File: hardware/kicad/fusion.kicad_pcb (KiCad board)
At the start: 2 copper layers, 32 parts, among them J1 BATTERY, J2 LSM6DSOX, J3 PICKIT, J4 HC-05, J5 FLEX, J7 FTDI, SW1 BUTTON, SW2 POWER, SW3 UART, U1 MCP1603, U2 PIC16F690

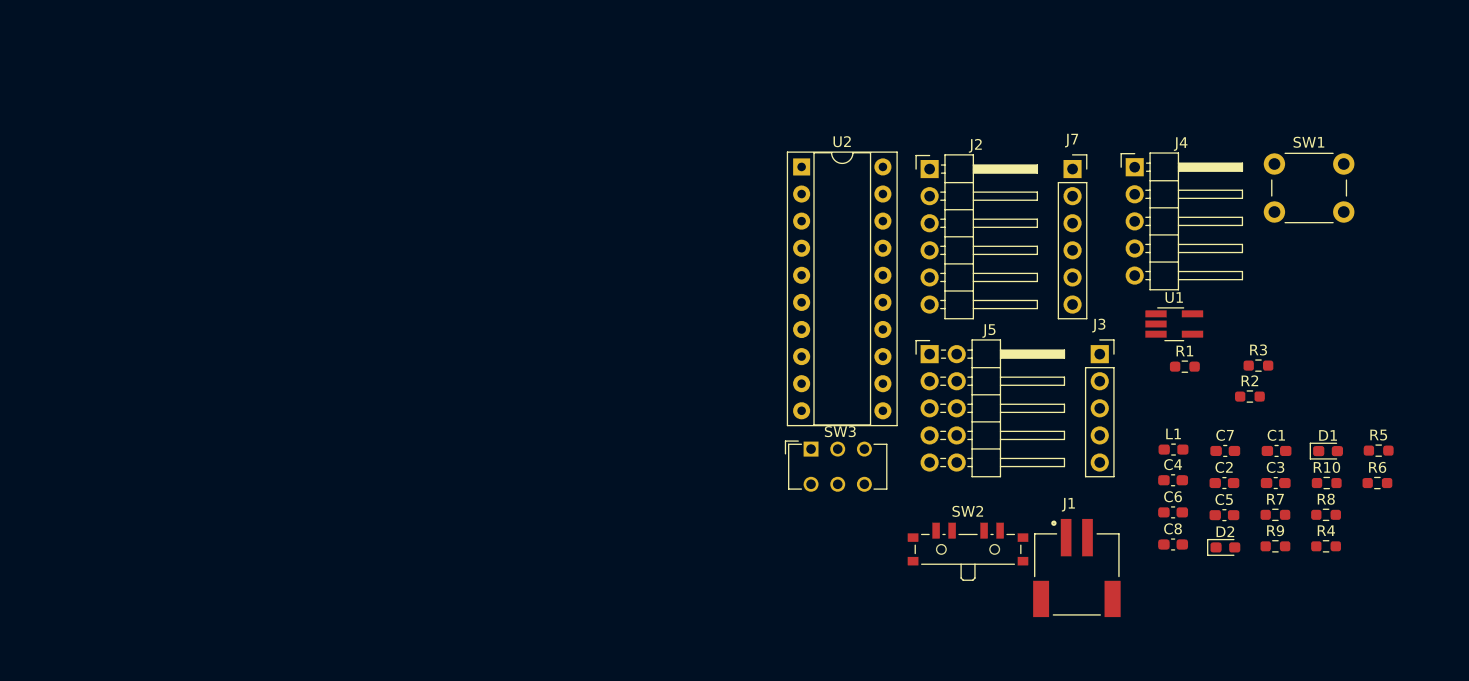
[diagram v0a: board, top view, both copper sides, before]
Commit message: Placing components
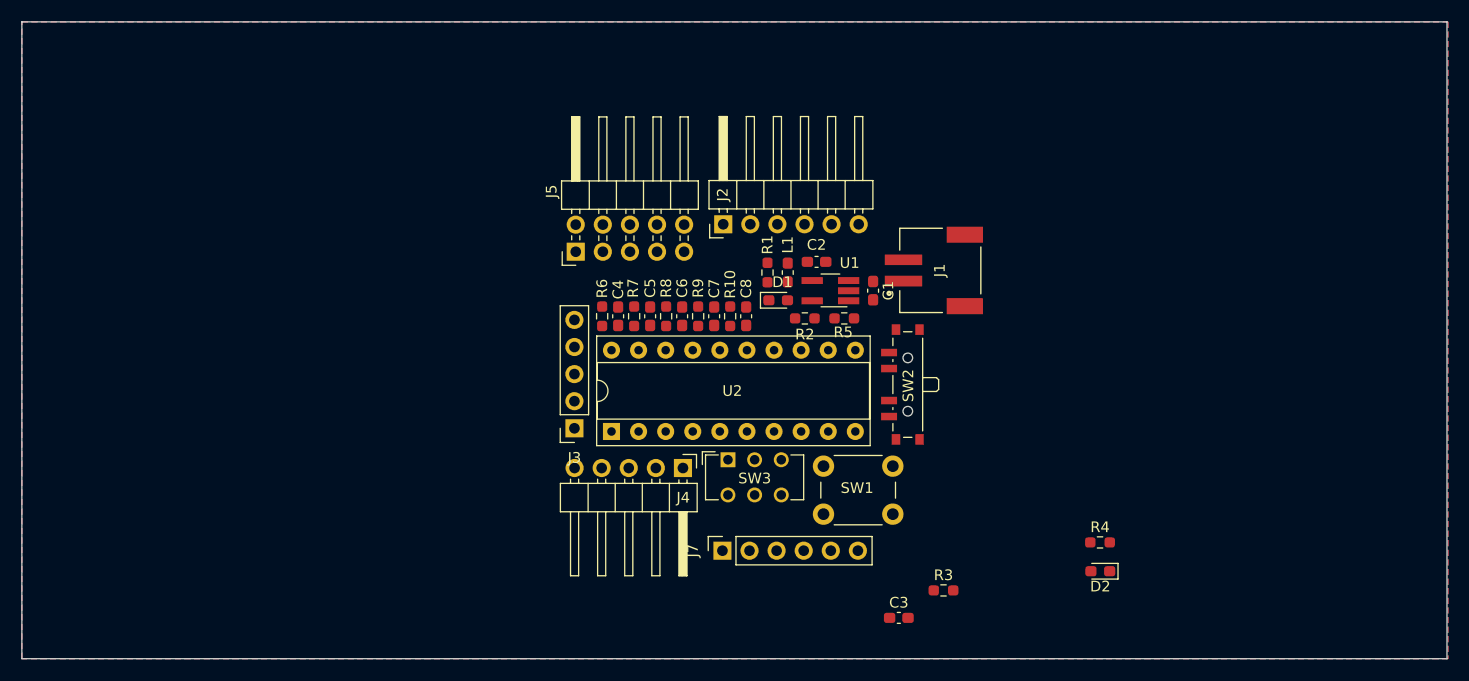
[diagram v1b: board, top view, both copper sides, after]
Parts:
- moved R6 74.3 mm to (143.0, 87.2), turned to -90 degrees
- moved R8 64.6 mm to (149.0, 87.2), turned to -90 degrees
- moved R7 62.9 mm to (146.0, 87.2), turned to -90 degrees
- moved R9 58.3 mm to (152.0, 87.2), turned to -90 degrees
- moved R10 58.1 mm to (155.0, 87.2), turned to -90 degrees
- moved C5 57.0 mm to (147.5, 87.2), turned to 90 degrees
- moved C4 54.2 mm to (144.5, 87.2), turned to 90 degrees
- moved D1 53.5 mm to (159.5, 85.7)
- moved R5 51.6 mm to (165.7, 87.4), turned to 180 degrees
- moved SW1 50.9 mm to (163.8, 101.2)
- moved J4 50.9 mm to (150.6, 101.4), turned to -90 degrees
- moved J3 49.7 mm to (140.4, 97.7), turned to 180 degrees
- moved C6 49.6 mm to (150.5, 87.2), turned to 90 degrees
- moved C7 49.6 mm to (153.5, 87.2), turned to 90 degrees
- moved J7 48.6 mm to (154.3, 109.2), turned to 90 degrees
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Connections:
- J5 pad 1: GNDREF -> THUMB
- J5 pad 10: THUMB -> GNDREF
- J5 pad 3: GNDREF -> INDEX
- J5 pad 5: GNDREF -> MIDDLE
- J5 pad 6: PINKY -> GNDREF
- J5 pad 8: MIDDLE -> GNDREF
- J5 pad 9: INDEX -> PINKY
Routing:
- added copper zone on B.Cu, net GNDREF
- added copper zone on F.Cu, net GNDREF
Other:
- board outline added: 133.6 x 59.7 mm
